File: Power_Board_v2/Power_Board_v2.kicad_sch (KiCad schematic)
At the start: 33 parts, among them J1 Conn_02x16_Odd_Even, Q1 MMBT5551L, U2 HUSB237-AA001-DN06R, U3 BQ24074RGT, U4 INA219AxDCN SOT-23

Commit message: misc.
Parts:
- C4, C8: LCSC (none) -> C19666; Supplier Part C19666 -> (none)
- C5, C6, C7: LCSC (none) -> C15849; Supplier Part C15849 -> (none)
- D1: LCSC (none) -> C2290; Supplier Part C2290 -> (none)
- D2: LCSC (none) -> C2286; Supplier Part C2286 -> (none)
- Q1: LCSC (none) -> C2145; Supplier Part C2145 -> (none)
- R10, R16: LCSC (none) -> C25804; Supplier Part C25804 -> (none)
- R11, R12, R13, R15, R18, R9: LCSC (none) -> C22843; Supplier Part C22843 -> (none)
- R14, R17: LCSC (none) -> C333100; Supplier Part C333100 -> (none)
- R2: LCSC (none) -> C23242; Supplier Part C19666 -> (none)
- R3: LCSC (none) -> C23159; Supplier Part C23159 -> (none)
- R4: LCSC (none) -> C17471
- R7: LCSC (none) -> C25804
- U2: LCSC (none) -> C22373734; SUPPLIER PART C22373734 -> (none)
- U3: LCSC (none) -> C54313; Supplier Part C54313 -> (none)
- U4: LCSC (none) -> C87469; Supplier Part C87469 -> (none)
- USBC1: LCSC (none) -> C165948; Supplier Part C165948 -> (none)
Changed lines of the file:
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@@
 			)
 		)
+		(property "LCSC" "C25804"
+			(at 195.58 60.96 0)
+			(effects
+				(font
+					(size 1.27 1.27)
+				)
+				(hide yes)
+			)
+		)
 		(pin "2"
 		)
@@
 			)
 		)
-		(property "Supplier Part" "C25804"
+		(property "LCSC" "C25804"
 			(at 71.12 40.64 0)
 			(effects
@@
 			)
 		)
-		(property "Supplier Part" "C22843"
+		(property "LCSC" "C22843"
 			(at 148.59 53.34 0)
 			(effects
@@
 			)
 		)
-		(property "Supplier Part" "C19666"
+		(property "LCSC" "C19666"
 			(at 190.5 58.42 0)
 			(effects
@@
 			)
 		)
-		(property "Supplier Part" "C165948"
+		(property "LCSC" "C165948"
 			(at 34.29 135.89 0)
 			(effects
@@
 			)
 		)
-		(property "Supplier Part" "C15849"
+		(property "LCSC" "C15849"
 			(at 148.59 27.94 0)
 			(effects
@@
 			)
 		)
-		(property "Supplier Part" "C22843"
+		(property "LCSC" "C22843"
 			(at 148.59 48.26 0)
 			(effects
@@
 			)
 		)
-		(property "Supplier Part" "C25804"
+		(property "LCSC" "C25804"
 			(at 71.12 64.77 0)
 			(effects
@@
 			)
 		)
-		(property "Supplier Part" "C87469"
+		(property "LCSC" "C87469"
 			(at 58.42 52.07 0)
 			(effects
@@
 			)
 		)
-		(property "Supplier Part" "C22843"
+		(property "LCSC" "C22843"
 			(at 157.48 88.9 0)
 			(effects
@@
 			)
 		)
-		(property "Supplier Part" "C2286"
+		(property "LCSC" "C2286"
 			(at 201.93 43.18 90)
 			(effects
@@
 			)
 		)
-		(property "Supplier Part" "C22843"
+		(property "LCSC" "C22843"
 			(at 201.93 35.56 0)
 			(effects
@@
 			)
 		)
+		(property "LCSC" "C17471"
+			(at 143.51 76.2 0)
+			(effects
+				(font
+					(size 1.27 1.27)
+				)
+				(hide yes)
+			)
+		)
 		(pin "2"
 		)
@@
 			)
 		)
-		(property "Supplier Part" " C2145"
+		(property "LCSC" " C2145"
 			(at 154.94 67.31 0)
 			(effects
@@
 			)
 		)
-		(property "SUPPLIER PART" "C22373734"
+		(property "LCSC" "C22373734"
 			(at 81.28 137.16 0)
 			(effects
@@
 			)
 		)
-		(property "Supplier Part" "C15849"
+		(property "LCSC" "C15849"
 			(at 78.74 54.61 0)
 			(effects
@@
 			)
 		)
-		(property "Supplier Part" "C23159"
+		(property "LCSC" "C23159"
 			(at 143.51 62.23 0)
 			(effects
@@
 			)
 		)
-		(property "Supplier Part" "C19666"
+		(property "LCSC" "C19666"
 			(at 218.44 39.37 0)
 			(effects
@@
 			)
 		)
-		(property "Supplier Part" "C15849"
+		(property "LCSC" "C15849"
 			(at 63.5 152.4 0)
 			(effects
@@
 			)
 		)
-		(property "Supplier Part" "C22843"
+		(property "LCSC" "C22843"
 			(at 210.82 35.56 0)
 			(effects
@@
 			)
 		)
-		(property "Supplier Part" "C22843"
+		(property "LCSC" "C22843"
 			(at 139.7 67.31 0)
 			(effects
@@
 			)
 		)
-		(property "Supplier Part" "C2290"
+		(property "LCSC" "C2290"
 			(at 210.82 43.18 90)
 			(effects
@@
 			)
 		)
-		(property "Supplier Part" "C333100"
+		(property "LCSC" "C333100"
 			(at 33.02 52.07 0)
 			(effects
@@
 			)
 		)
-		(property "Supplier Part" "C333100"
+		(property "LCSC" "C333100"
 			(at 39.37 52.07 0)
 			(effects
@@
 			)
 		)
-		(property "Supplier Part" "C19666"
+		(property "LCSC" "C23242"
 			(at 71.12 152.4 0)
 			(effects
@@
 			)
 		)
-		(property "Supplier Part" "C54313"
+		(property "LCSC" "C54313"
 			(at 173.99 40.64 90)
 			(effects

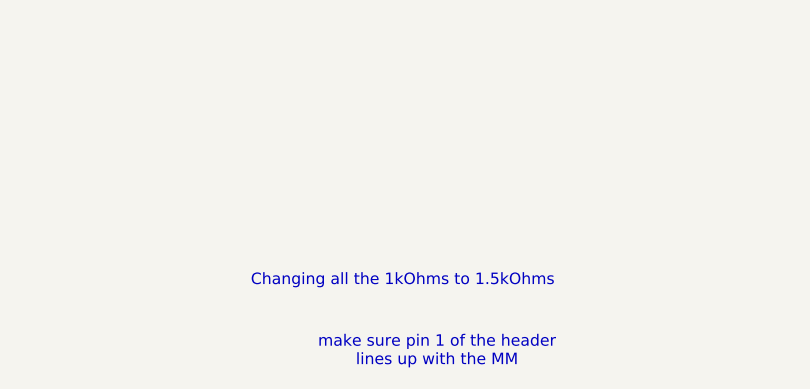
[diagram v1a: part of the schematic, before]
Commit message: Test
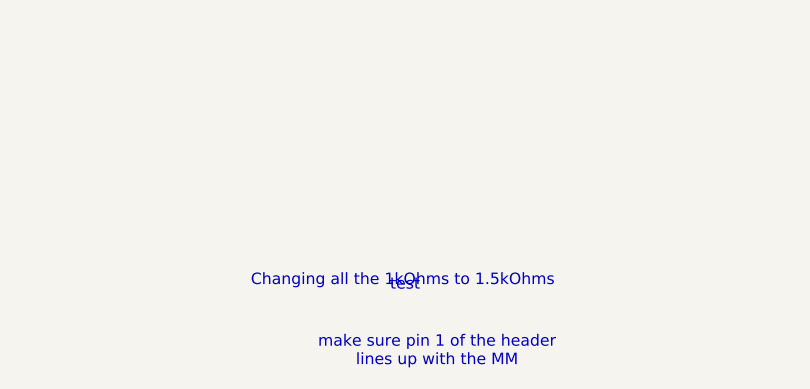
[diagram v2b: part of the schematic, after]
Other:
- note added: "test"
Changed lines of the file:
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@@
+		)
+	)
+	(text "test\n"
+		(exclude_from_sim no)
+		(at 267.97 260.35 0)
+		(effects
+			(font
+				(size 1.27 1.27)
+			)
 		)
 	)
